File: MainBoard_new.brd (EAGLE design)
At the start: 60 parts, among them T1 BC847, U1 STM32F10XRXT6, Y1 8MHz, Y2 32.768kHz

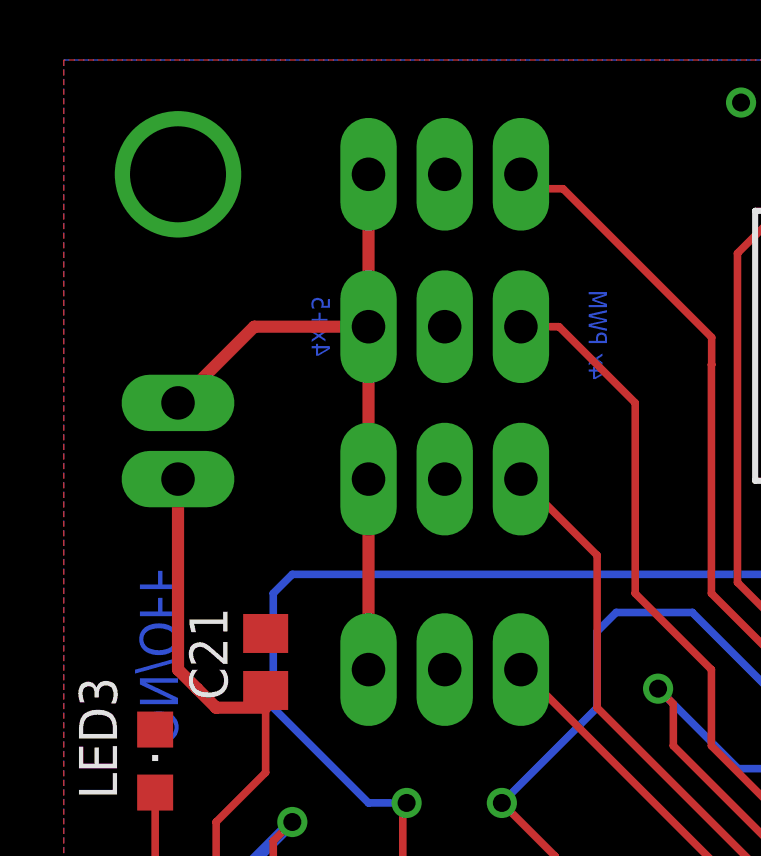
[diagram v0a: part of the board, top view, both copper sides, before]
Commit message: poprawki płytki, kodzik
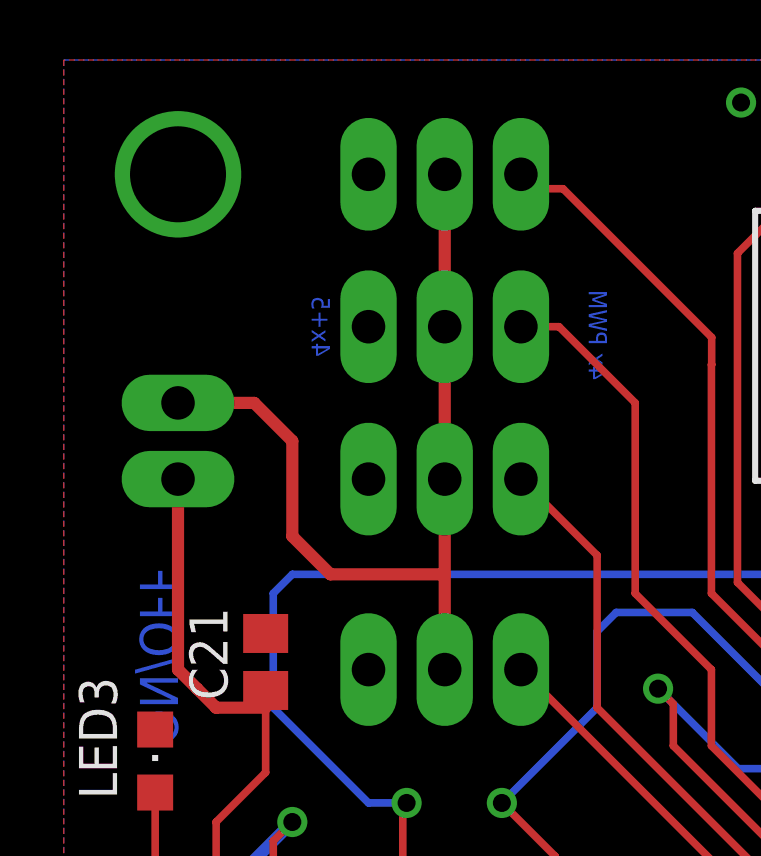
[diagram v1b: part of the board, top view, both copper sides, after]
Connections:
- net 5V: now also JP5.2, JP6.2, JP7.2, JP8.2; no longer JP5.1, JP6.1, JP7.1, JP8.1
- net GND: now also JP5.1, JP6.1, JP7.1, JP8.1; no longer JP5.2, JP6.2, JP7.2, JP8.2
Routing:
- net 5V: track 23.9 -> 29.6 mm
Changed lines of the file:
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@@
 <setting verticaltext="up"/>
 </settings>
-<grid distance="0" unitdist="inch" unit="inch" style="lines" multiple="1" display="yes" altdistance="0.025" altunitdist="inch" altunit="inch"/>
+<grid distance="0.025" unitdist="inch" unit="inch" style="lines" multiple="1" display="yes" altdistance="0.025" altunitdist="inch" altunit="inch"/>
 <layers>
-<layer number="1" name="Top" color="4" fill="1" visible="no" active="yes"/>
+<layer number="1" name="Top" color="4" fill="1" visible="yes" active="yes"/>
 <layer number="2" name="Route2" color="1" fill="3" visible="no" active="no"/>
 <layer number="3" name="Route3" color="4" fill="3" visible="no" active="no"/>
@@
 <contactref element="IC3" pad="1"/>
 <wire x1="20.88" y1="38.72" x2="20.88" y2="37.39" width="0.3048" layer="1"/>
-<contactref element="JP5" pad="2"/>
-<contactref element="JP6" pad="2"/>
-<contactref element="JP7" pad="2"/>
-<contactref element="JP8" pad="2"/>
 <wire x1="41.2595" y1="42.819" x2="41.041" y2="42.819" width="0.254" layer="16"/>
 <wire x1="41.041" y1="42.819" x2="40.767" y2="42.545" width="0.254" layer="16"/>
@@
 <contactref element="SG1" pad="+"/>
 <via x="12.417934375" y="58.27184375" extent="1-16" drill="0.6" shape="square"/>
+<contactref element="JP6" pad="1"/>
+<contactref element="JP7" pad="1"/>
+<contactref element="JP8" pad="1"/>
+<contactref element="JP5" pad="1"/>
 </signal>
 <signal name="SWDIO">
@@
 </signal>
 <signal name="5V">
-<contactref element="JP5" pad="1"/>
-<contactref element="JP6" pad="1"/>
-<contactref element="JP7" pad="1"/>
-<contactref element="JP8" pad="1"/>
 <contactref element="JP9" pad="1"/>
-<wire x1="0" y1="55.88" x2="0" y2="50.8" width="0.4064" layer="1"/>
-<wire x1="0" y1="50.8" x2="0" y2="45.72" width="0.4064" layer="1"/>
-<wire x1="0" y1="45.72" x2="0" y2="39.37" width="0.4064" layer="1"/>
-<wire x1="0" y1="50.8" x2="-3.81" y2="50.8" width="0.4064" layer="1"/>
-<wire x1="-3.81" y1="50.8" x2="-6.35" y2="48.26" width="0.4064" layer="1"/>
+<contactref element="JP5" pad="2"/>
+<contactref element="JP6" pad="2"/>
+<contactref element="JP7" pad="2"/>
+<contactref element="JP8" pad="2"/>
+<wire x1="2.54" y1="39.37" x2="2.54" y2="42.545" width="0.4064" layer="1"/>
+<wire x1="2.54" y1="42.545" x2="2.54" y2="45.72" width="0.4064" layer="1"/>
+<wire x1="2.54" y1="45.72" x2="2.54" y2="50.8" width="0.4064" layer="1"/>
+<wire x1="2.54" y1="50.8" x2="2.54" y2="55.88" width="0.4064" layer="1"/>
+<wire x1="-6.35" y1="48.26" x2="-3.81" y2="48.26" width="0.4064" layer="1"/>
+<wire x1="-3.81" y1="48.26" x2="-2.54" y2="46.99" width="0.4064" layer="1"/>
+<wire x1="-2.54" y1="46.99" x2="-2.54" y2="43.815" width="0.4064" layer="1"/>
+<wire x1="-2.54" y1="43.815" x2="-1.27" y2="42.545" width="0.4064" layer="1"/>
+<wire x1="-1.27" y1="42.545" x2="2.54" y2="42.545" width="0.4064" layer="1"/>
 </signal>
 <signal name="REG1">
